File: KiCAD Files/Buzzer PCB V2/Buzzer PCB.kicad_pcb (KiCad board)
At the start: 2 copper layers, 147.8 x 93.4 mm, 26 parts, among them J1 2600mAh LiPo JST-PH bottom, J10 SparkFun Thing Plus ESP32 WRO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, J11 M16968 OLED + Rotary Knob, J5 HGLRC M100 Mini GPS, J6 BMP581/BMP5xx top pads, J7 SHT41 top pads, Q1 S8050, Q2 S8050, Q3 S8050, SW1 SS12D00G5 power switch, U1 TP4057 USB-C charger, U2 Comidox 5V Booster

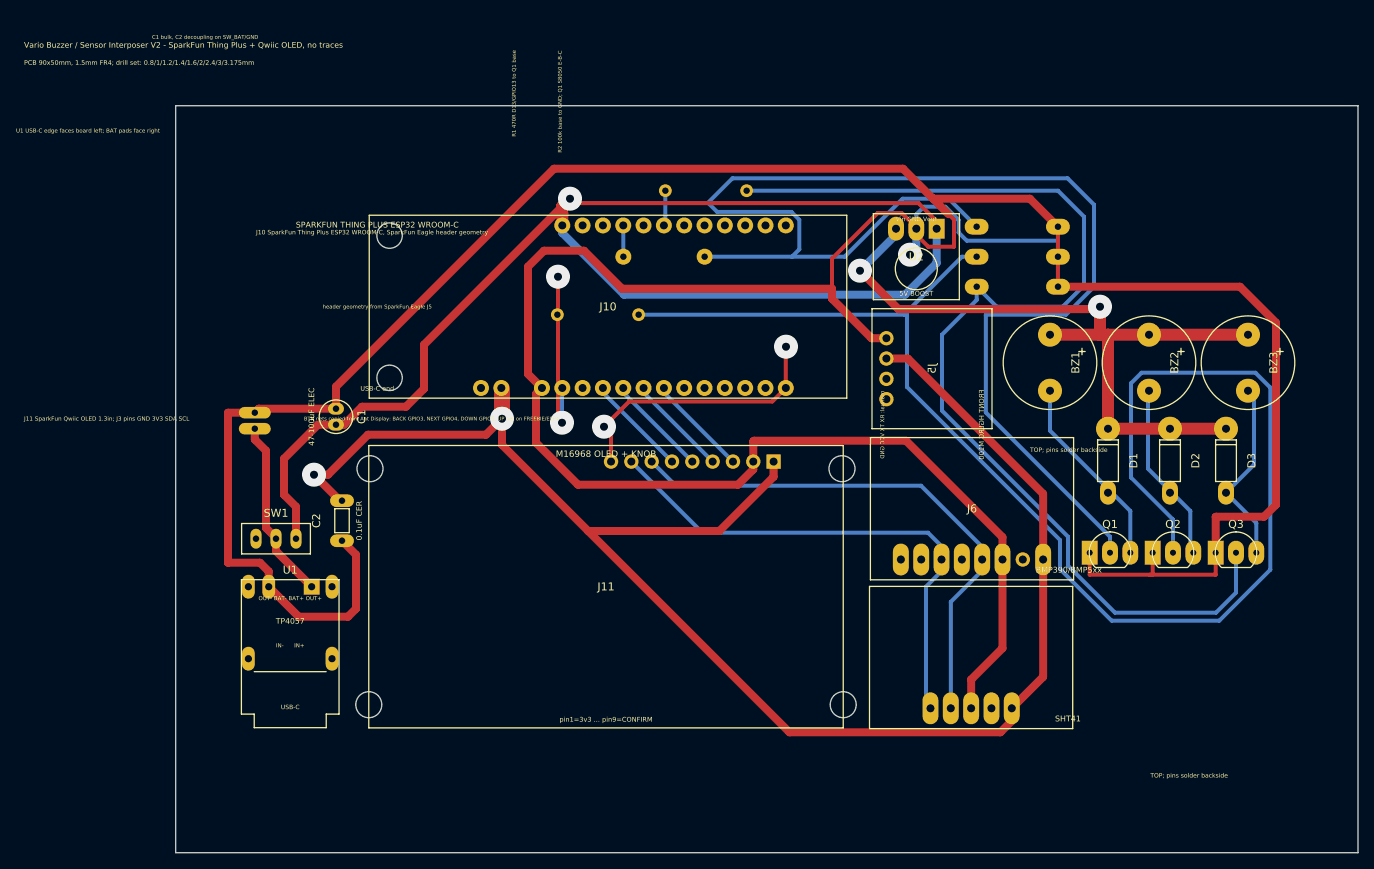
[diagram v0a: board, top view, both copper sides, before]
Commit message: final routing
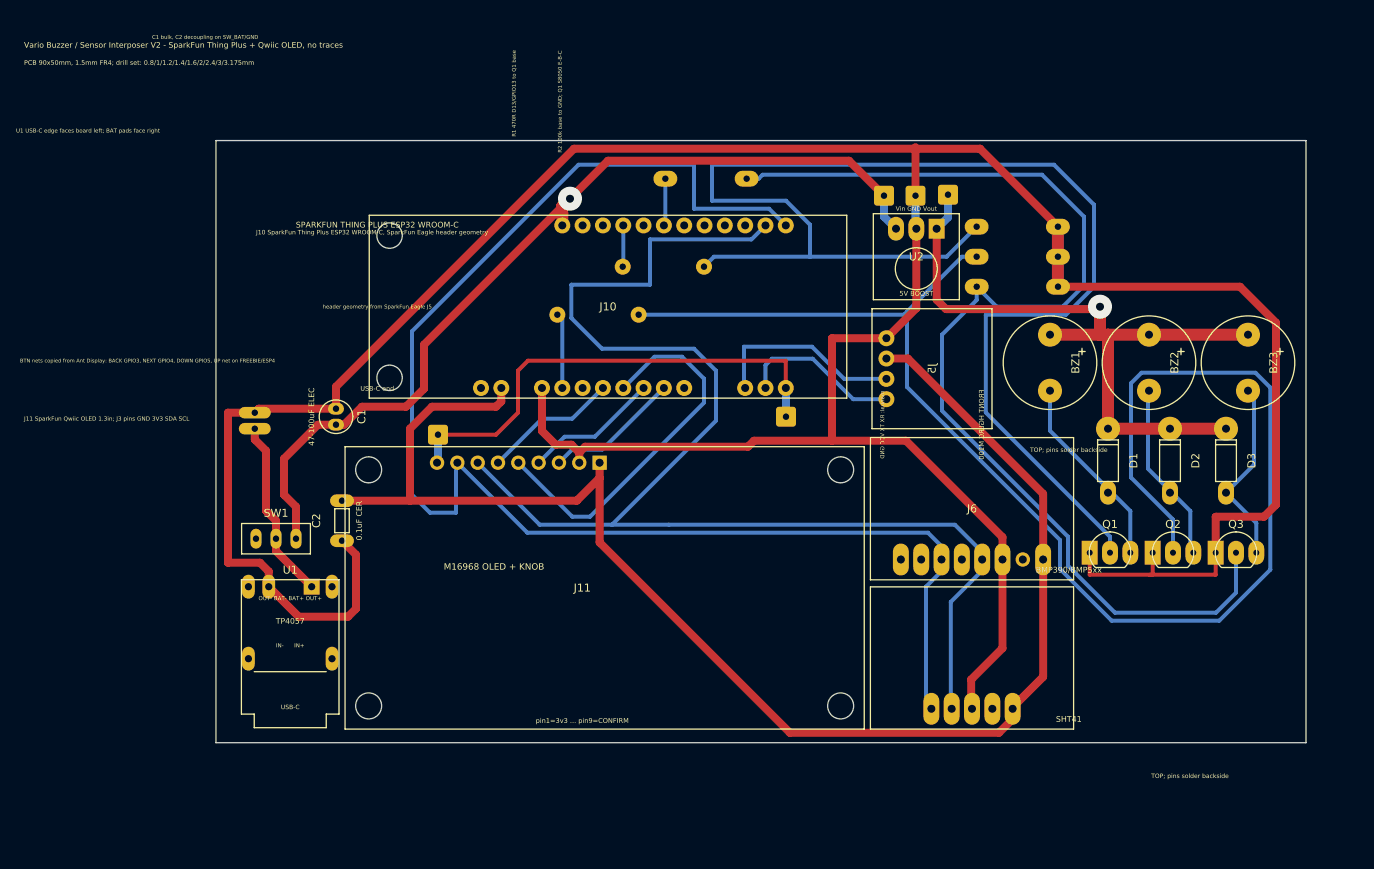
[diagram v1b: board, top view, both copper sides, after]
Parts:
- added ?: , , F.Cu at (133.2, 82.0)
- added ?: , , F.Cu at (149.4, 54.4)
- added ?: , , F.Cu at (89.8, 84.2)
- added ?: , , F.Cu at (145.5, 54.4)
- added REF**: SolderWire-0.127sqmm_1x01_D0.48mm_OD1mm, Connector_Wire:SolderWire-0.127sqmm_1x01_D0.48mm_OD1mm, F.Cu at (153.5, 54.2)
- moved J11 37.0 mm to (78.1, 85.8)
- moved R3 1.50 mm to (128.3, 52.2)
- moved R1 1.25 mm to (123.0, 63.2)
- moved J7 0.13 mm to (156.5, 112.2)
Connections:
- U2 pad 1: /SW_BAT -> /BOOST_5V
- U2 pad 3: /BOOST_5V -> /SW_BAT
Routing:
- net /SDA: track 64.4 -> 181.0 mm
- net /SCL: track 67.5 -> 169.1 mm
- net /GND: track 496.4 -> 422.2 mm, vias 1 -> 0
- net /SW_BAT: track 171.6 -> 115.4 mm
- net /BTN_DOWN_GPIO5: track 12.8 -> 47.8 mm
- net /OLED_CONFIRM: track 34.6 -> 60.9 mm, vias 2 -> 0
- net /GPS_TX_THING_RX: track 0.15 -> 24.7 mm
- net /GPS_RX_THING_TX: track 0.00 -> 20.4 mm
- net /BUZZER2_ESP26: track 27.8 -> 9.58 mm, vias 2 -> 0
- net /3V3: track 202.1 -> 185.7 mm, vias 2 -> 0
- net /BTN_UP_GPIO21: track 12.8 -> 17.0 mm
- net /BTN_NEXT_GPIO4: track 12.8 -> 17.0 mm
- net /BTN_BACK_GPIO3: track 12.8 -> 17.0 mm
- net /BOOST_5V: track 94.1 -> 90.5 mm, vias 2 -> 1
- net /BUZZER3_GPIO2_ESP27: track 4.42 -> 5.92 mm
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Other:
- board size 147.8 x 93.4 mm -> 136.3 x 75.3 mm
